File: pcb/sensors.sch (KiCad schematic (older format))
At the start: 13 parts, among them J2 Conn_01x04_Male, Q2 BSS138DW-7-F, U4 BME280, U6 SGP30, U7 TSL2591

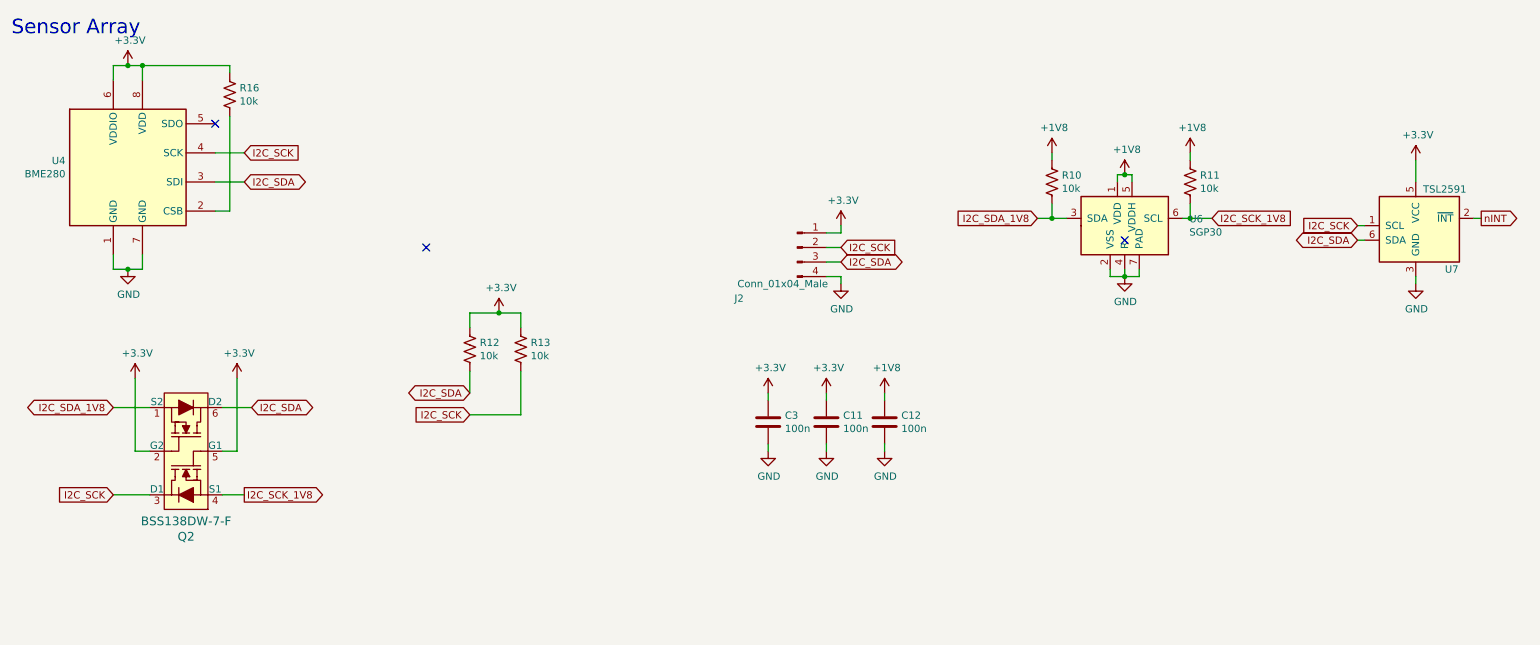
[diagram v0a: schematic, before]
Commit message: add gerbers for room monitor v1
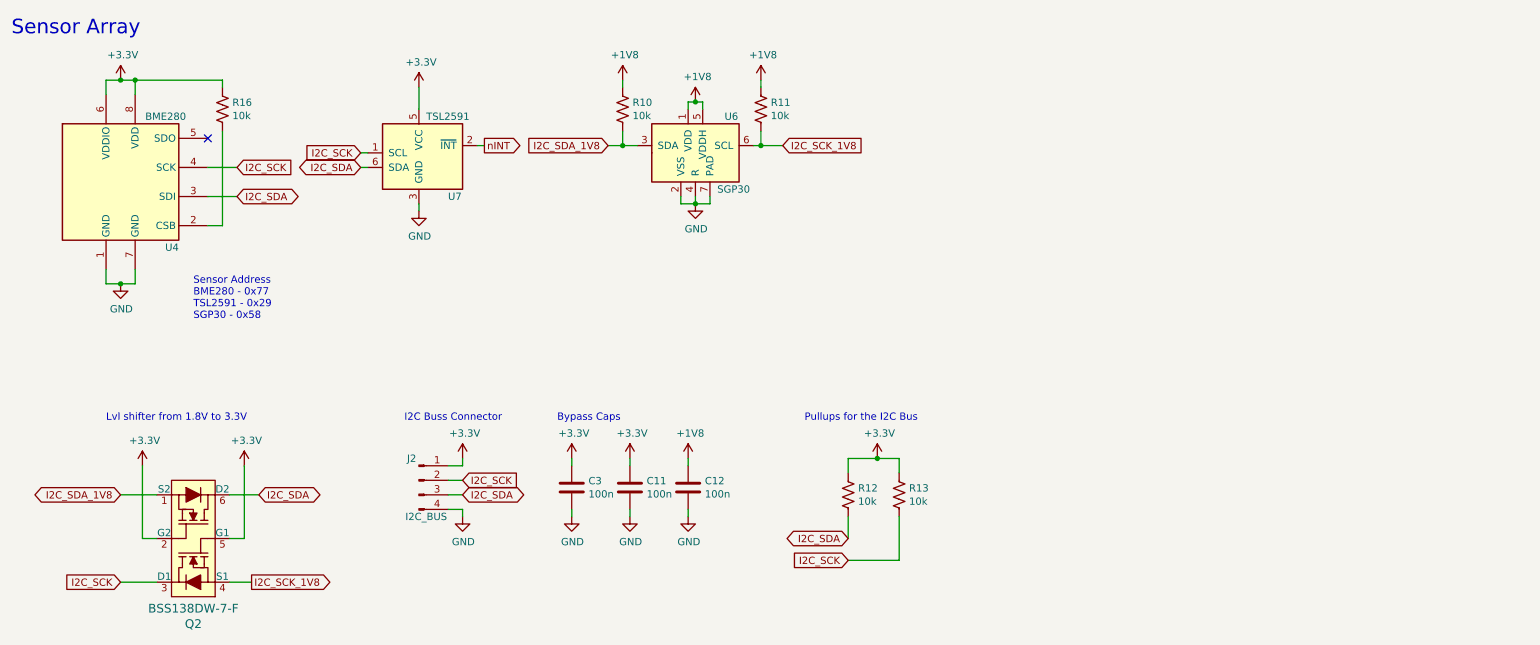
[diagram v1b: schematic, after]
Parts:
- J2: value Conn_01x04_Male -> I2C_BUS
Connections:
- no-connect marks 3 -> 1
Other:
- note added: "Bypass Caps"
- note added: "I2C Buss Connector"
- note added: "Lvl shifter from 1.8V to 3.3V"
- note added: "Pullups for the I2C Bus"
- note added: "Sensor Address\nBME280 - 0x77\nTSL2591 - 0x29\nSGP30 - 0x58"
- moved on the sheet: C11, C12, C3, J2, Q2, R10, R11, R12, R13, R16, U4, U6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
